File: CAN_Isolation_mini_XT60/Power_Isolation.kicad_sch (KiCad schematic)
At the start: 13 parts, among them J1 S4B-XH-A, U3 MGS3123R3, U4 MGS1R51205, U5 TVS1800DRVR, U7 MGS102405

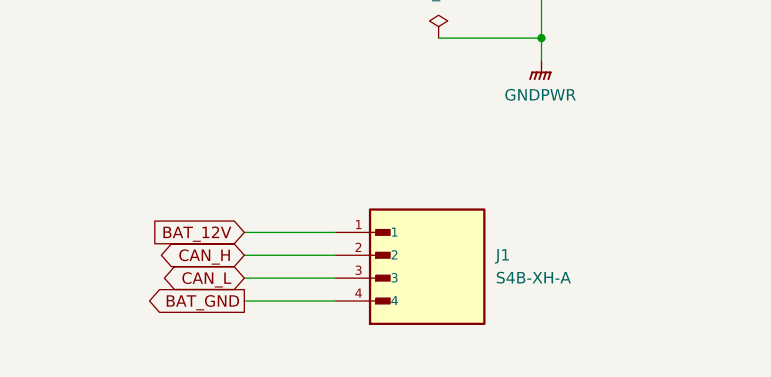
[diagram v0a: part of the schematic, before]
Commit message: Change connector.
Change connector.
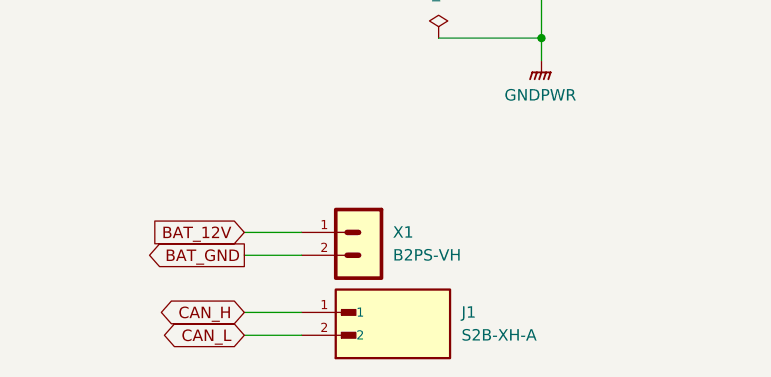
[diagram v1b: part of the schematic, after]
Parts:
- removed J1: S4B-XH-A, CAN_Isolation:JST_S4B-XH-A, symbol S4B-XH-A:S4B-XH-A
- added J1: S2B-XH-A, CAN_Isolation:JST_S2B-XH-A, symbol S2B-XH-A:S2B-XH-A
- added X1: B2PS-VH, CAN_Isolation:B2PS-VH, symbol B2PS-VH:B2PS-VH
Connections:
- net +12V: now also X1.1
- net CAN_H: now also J1.1
- net CAN_L: now also J1.2
- net GNDPWR: now also X1.2
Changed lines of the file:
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@@
+	(wire
+		(pts
+			(xy 43.18 173.99) (xy 49.53 173.99)
+		)
+		(stroke
+			(width 0)
+			(type default)
+		)
+	)
 	(wire
 		(pts
@@
 	(wire
 		(pts
+			(xy 43.18 162.56) (xy 49.53 162.56)
+		)
+		(stroke
+			(width 0)
+			(type default)
+		)
+	)
+	(wire
+		(pts
 			(xy 78.74 133.35) (xy 81.28 133.35)
 		)
@@
 	(wire
 		(pts
-			(xy 43.18 167.64) (xy 53.34 167.64)
-		)
-		(stroke
-			(width 0)
-			(type default)
-		)
-	)
-	(wire
-		(pts
 			(xy 162.56 140.97) (xy 173.99 140.97)
 		)
@@
 	(wire
 		(pts
-			(xy 43.18 170.18) (xy 53.34 170.18)
-		)
-		(stroke
-			(width 0)
-			(type default)
-		)
-	)
-	(wire
-		(pts
 			(xy 76.2 140.97) (xy 76.2 143.51)
 		)
@@
 	(wire
 		(pts
-			(xy 43.18 162.56) (xy 53.34 162.56)
+			(xy 43.18 165.1) (xy 49.53 165.1)
 		)
 		(stroke
@@
 	(wire
 		(pts
-			(xy 43.18 165.1) (xy 53.34 165.1)
-		)
-		(stroke
-			(width 0)
-			(type default)
-		)
-	)
-	(wire
-		(pts
 			(xy 114.3 53.34) (xy 121.92 53.34)
 		)
@@
 		(pts
 			(xy 121.92 55.88) (xy 121.92 60.96)
+		)
+		(stroke
+			(width 0)
+			(type default)
+		)
+	)
+	(wire
+		(pts
+			(xy 43.18 171.45) (xy 49.53 171.45)
 		)
 		(stroke
@@
 	(global_label "CAN_H"
 		(shape bidirectional)
-		(at 43.18 165.1 180)
+		(at 43.18 171.45 180)
 		(fields_autoplaced yes)
 		(effects
@@
 		)
 		(property "Intersheetrefs" "${INTERSHEET_REFS}"
-			(at 33.0963 165.1 0)
+			(at 33.0963 171.45 0)
 			(effects
 				(font
@@
 	(global_label "BAT_GND"
 		(shape output)
-		(at 43.18 170.18 180)
+		(at 43.18 165.1 180)
 		(fields_autoplaced yes)
 		(effects
@@
 		)
 		(property "Intersheetrefs" "${INTERSHEET_REFS}"
-			(at 32.0305 170.18 0)
+			(at 32.0305 165.1 0)
 			(effects
 				(font
@@
 	(global_label "CAN_L"
 		(shape bidirectional)
-		(at 43.18 167.64 180)
+		(at 43.18 173.99 180)
 		(fields_autoplaced yes)
 		(effects
@@
 		)
 		(property "Intersheetrefs" "${INTERSHEET_REFS}"
-			(at 33.3987 167.64 0)
+			(at 33.3987 173.99 0)
 			(effects
 				(font
@@
 	)
 	(symbol
+		(lib_id "B2PS-VH:B2PS-VH")
+		(at 57.15 165.1 180)
+		(unit 1)
+		(exclude_from_sim no)
+		(in_bom yes)
+		(on_board yes)
+		(dnp no)
+		(fields_autoplaced yes)
+		(property "Reference" "X1"
+			(at 59.69 162.5599 0)
+			(effects
+				(font
+					(size 1.27 1.27)
+				)
+				(justify right)
+			)
+		)
+		(property "Value" "B2PS-VH"
+			(at 59.69 165.0999 0)
+			(effects
+				(font
+					(size 1.27 1.27)
+				)
+				(justify right)
+			)
+		)
+		(property "Footprint" "CAN_Isolation:B2PS-VH"
+			(at 57.15 165.1 0)
+			(effects
+				(font
+					(size 1.27 1.27)
+				)
+				(justify bottom)
+				(hide yes)
+			)
+		)
+		(property "Datasheet" ""
+			(at 57.15 165.1 0)
+			(effects
+				(font
+					(size 1.27 1.27)
+				)
+				(hide yes)
+			)
+		)
+		(property "Description" ""
+			(at 57.15 165.1 0)
+			(effects
+				(font
+					(size 1.27 1.27)
+				)
+				(hide yes)
+			)
+		)
+		(property "MF" "JST Sales"
+			(at 57.15 165.1 0)
+			(effects
+				(font
+					(size 1.27 1.27)
+				)
+				(justify bottom)
+				(hide yes)
+			)
+		)
+		(property "Description_1" "Connector Header Through Hole, Right Angle 2 position 0.156 (3.96mm)"
+			(at 57.15 165.1 0)
+			(effects
+				(font
+					(size 1.27 1.27)
+				)
+				(justify bottom)
+				(hide yes)
+			)
+		)
+		(property "Package" "None"
+			(at 57.15 165.1 0)
+			(effects
+				(font
+					(size 1.27 1.27)
+				)
+				(justify bottom)
+				(hide yes)
+			)
+		)
+		(property "Price" "None"
+			(at 57.15 165.1 0)
+			(effects
+				(font
+					(size 1.27 1.27)
+				)
+				(justify bottom)
+				(hide yes)
+			)
+		)
+		(property "SnapEDA_Link" "https://www.snapeda.com/parts/B2PS-VH/JST/view-part/?ref=snap"
+			(at 57.15 165.1 0)
+			(effects
+				(font
+					(size 1.27 1.27)
+				)
+				(justify bottom)
+				(hide yes)
+			)
+		)
+		(property "MP" "B2PS-VH"
+			(at 57.15 165.1 0)
+			(effects
+				(font
+					(size 1.27 1.27)
+				)
+				(justify bottom)
+				(hide yes)
+			)
+		)
+		(property "Availability" "In Stock"
+			(at 57.15 165.1 0)
+			(effects
+				(font
+					(size 1.27 1.27)
+				)
+				(justify bottom)
+				(hide yes)
+			)
+		)
+		(property "Check_prices" "https://www.snapeda.com/parts/B2PS-VH/JST/view-part/?ref=eda"
+			(at 57.15 165.1 0)
+			(effects
+				(font
+					(size 1.27 1.27)
+				)
+				(justify bottom)
+				(hide yes)
+			)
+		)
+		(pin "1"
+		)
+		(pin "2"
+		)
+		(instances
+			(project ""
+				(path "/d188d587-a283-4d42-bf18-6e85dcc02a49/7e4d328d-cac9-4e09-9774-03494cf924e9"
+					(reference "X1")
+					(unit 1)
+				)
+			)
+		)
+	)
+	(symbol
 		(lib_id "SMLD12EN1WT86:SMLD12EN1WT86")
 		(at 189.23 85.09 270)
@@
 	)
 	(symbol
-		(lib_id "S4B-XH-A:S4B-XH-A")
-		(at 63.5 167.64 0)
-		(unit 1)
-		(exclude_from_sim no)
-		(in_bom yes)
-		(on_board yes)
-		(dnp no)
-		(property "Reference" "J1"
-			(at 71.12 165.0999 0)
-			(effects
-				(font
-					(size 1.27 1.27)
-				)
-				(justify left)
-			)
-		)
-		(property "Value" "S4B-XH-A"
-			(at 71.12 167.6399 0)
-			(effects
-				(font
-					(size 1.27 1.27)
-				)
-				(justify left)
-			)
-		)
-		(property "Footprint" "CAN_Isolation:JST_S4B-XH-A"
-			(at 63.5 167.64 0)
-			(effects
-				(font
-					(size 1.27 1.27)
-				)
-				(justify bottom)
-				(hide yes)
-			)
-		)
-		(property "Datasheet" ""
-			(at 63.5 167.64 0)
-			(effects
-				(font
-					(size 1.27 1.27)
-				)
-				(hide yes)
-			)
-		)
-		(property "Description" ""
-			(at 63.5 167.64 0)
-			(effects
-				(font
-					(size 1.27 1.27)
-				)
-				(hide yes)
-			)
-		)
-		(property "MANUFACTURER" "JST"
-			(at 63.5 167.64 0)
-			(effects
-				(font
-					(size 1.27 1.27)
-				)
-				(justify bottom)
-				(hide yes)
-			)
-		)
-		(pin "1"
-		)
-		(pin "2"
-		)
-		(pin "3"
-		)
-		(pin "4"
-		)
-		(instances
-			(project ""
-				(path "/d188d587-a283-4d42-bf18-6e85dcc02a49/7e4d328d-cac9-4e09-9774-03494cf924e9"
-					(reference "J1")
-					(unit 1)
-				)
-			)
-		)
-	)
-	(symbol
 		(lib_id "power:PWR_FLAG")
 		(at 173.99 140.97 0)
@@
 					(unit 1)
 				)
+			)
+		)
+	)
+	(symbol
+		(lib_id "S2B-XH-A:S2B-XH-A")
+		(at 59.69 173.99 0)
+		(unit 1)
+		(exclude_from_sim no)
+		(in_bom yes)
+		(on_board yes)
+		(dnp no)
+		(fields_autoplaced yes)
+		(property "Reference" "J1"
+			(at 67.31 171.4499 0)
+			(effects
+				(font
+					(size 1.27 1.27)
+				)
+				(justify left)
+			)
+		)
+		(property "Value" "S2B-XH-A"
+			(at 67.31 173.9899 0)
+			(effects
+				(font
+					(size 1.27 1.27)
+				)
+				(justify left)
+			)
+		)
+		(property "Footprint" "CAN_Isolation:JST_S2B-XH-A"
+			(at 59.69 173.99 0)
+			(effects
+				(font
+					(size 1.27 1.27)
+				)
+				(justify bottom)
+				(hide yes)
+			)
+		)
+		(property "Datasheet" ""
+			(at 59.69 173.99 0)
+			(effects
+				(font
+					(size 1.27 1.27)
+				)
+				(hide yes)
+			)
+		)
+		(property "Description" ""
+			(at 59.69 173.99 0)
+			(effects
+				(font
+					(size 1.27 1.27)
+				)
+				(hide yes)
+			)
+		)
+		(property "MANUFACTURER" "JST"
+			(at 59.69 173.99 0)
+			(effects
+				(font
+					(size 1.27 1.27)
+				)
+				(justify bottom)
+				(hide yes)
+			)
+		)
+		(pin "2"
+		)
+		(pin "1"
+		)
+		(instances
+			(project "CAN_Isolation_mini"
+				(path "/d188d587-a283-4d42-bf18-6e85dcc02a49/7e4d328d-cac9-4e09-9774-03494cf924e9"
+					(reference "J1")
+					(unit 1)
+				)
